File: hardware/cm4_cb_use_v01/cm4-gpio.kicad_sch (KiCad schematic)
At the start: 16 parts, among them J1 DNP, J4 molex_5046_2pin, J5 TPS62133RGTR, U1 SN74LVC1G07DCKR

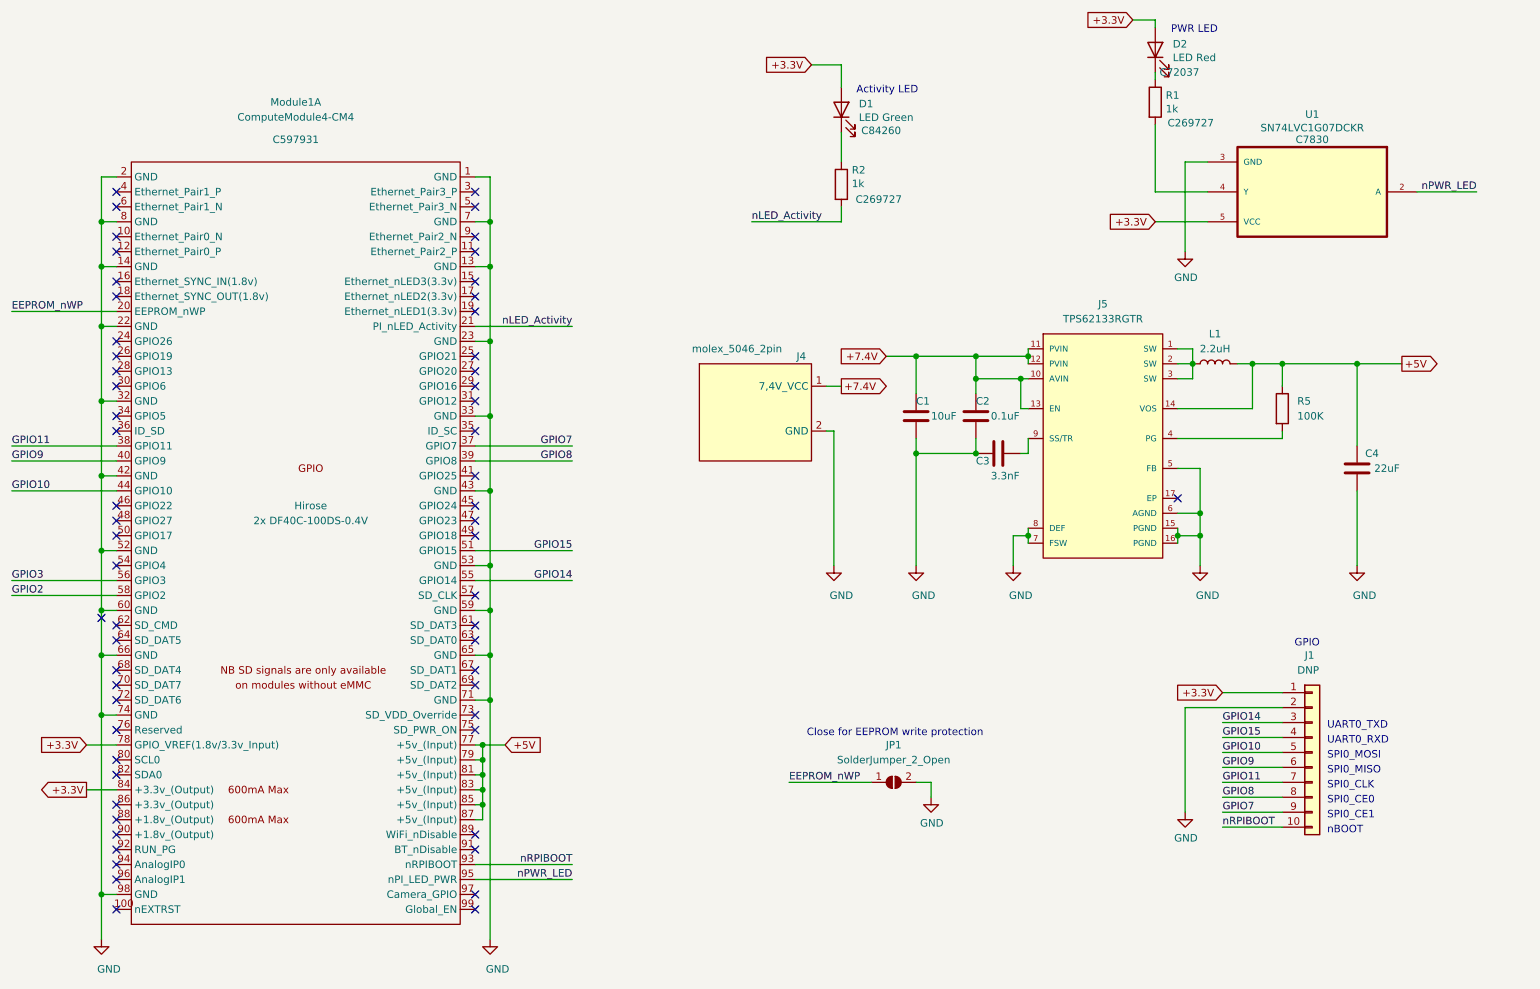
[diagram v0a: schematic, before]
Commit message: updated
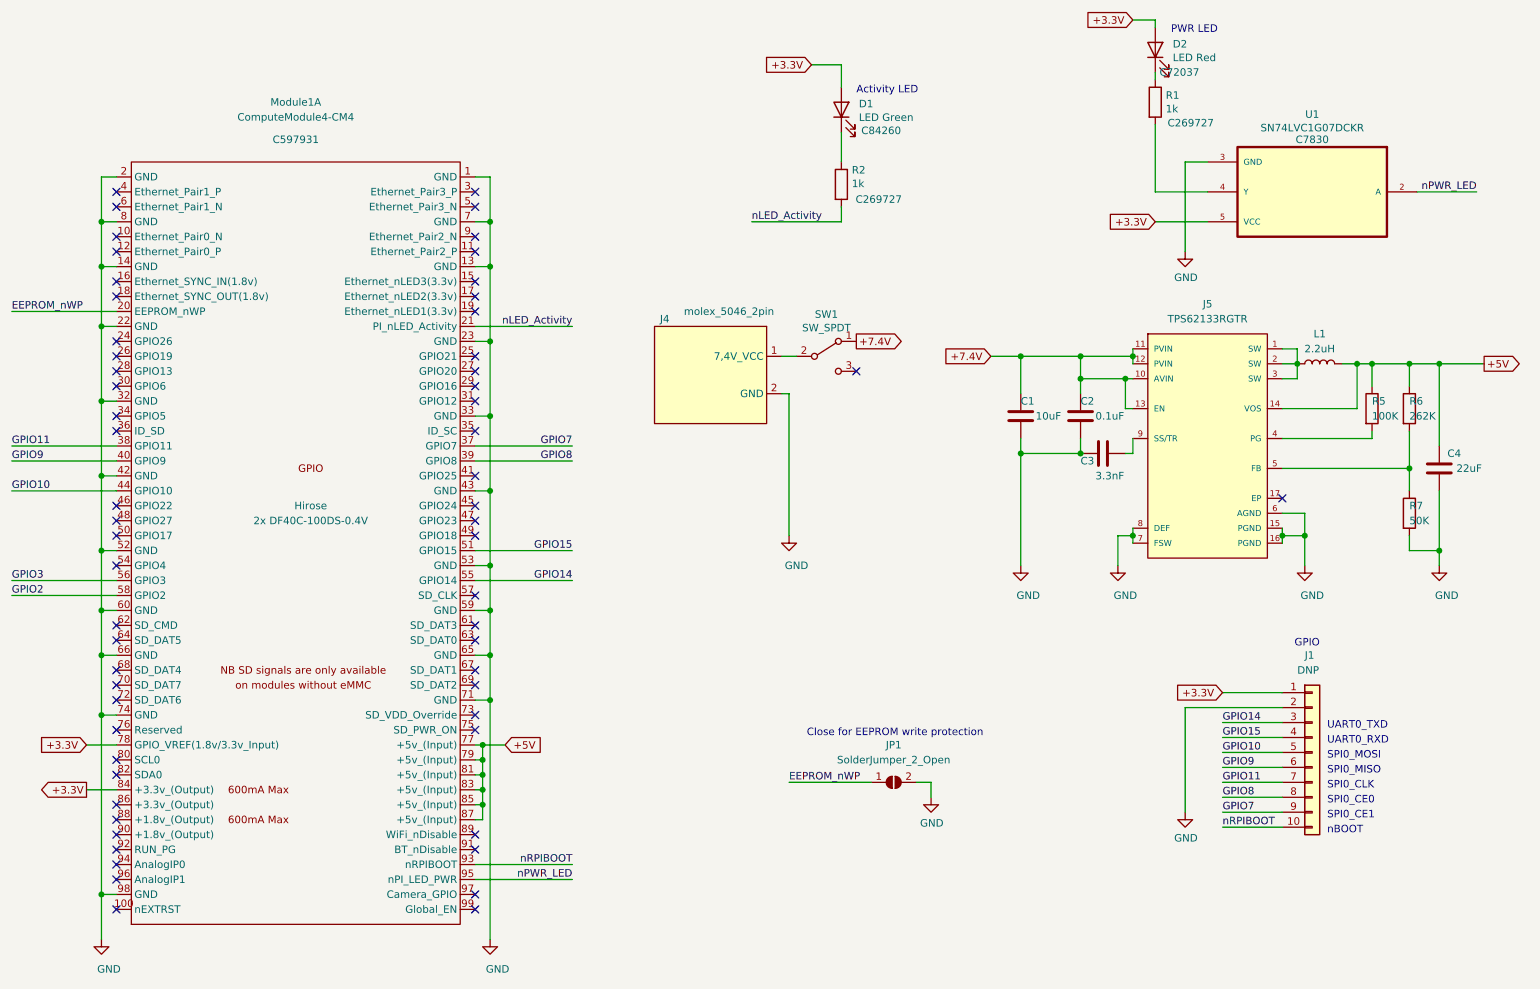
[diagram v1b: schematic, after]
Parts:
- added R6: 262K, Resistor_SMD:R_0805_2012Metric, symbol Device:R
- added R7: 50K, Resistor_SMD:R_0805_2012Metric, symbol Device:R
- added SW1: SW_SPDT, c&k_slide_switch_1101M2S3AQE2:c&k_slide_switch_1101M2S3AQE2, symbol Switch:SW_SPDT
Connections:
- net +5V: now also R6.1
- net +7.4V: now also SW1.1 (A); no longer J4.1 (7,4V_VCC)
- net GND: now also R7.2; no longer J5.5 (FB)
- new net: J5.5 (FB), R6.2, R7.1
- new net: J4.1 (7,4V_VCC), SW1.2 (B)
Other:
- moved on the sheet: C1, C2, C3, C4, J4, J5, L1, R5
